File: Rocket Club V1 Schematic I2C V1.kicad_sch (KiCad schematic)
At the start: 8 parts, among them IC1 STM32H573RIT6, J1 USB4135-GF-A_REVA, U1 H3LIS100DLTR, U2 LSM6DSOTR, U3 MAX-M8W-0, U4 MT25TL01GBBB8ESF-0AAT, U5 STLINK-V3MODS

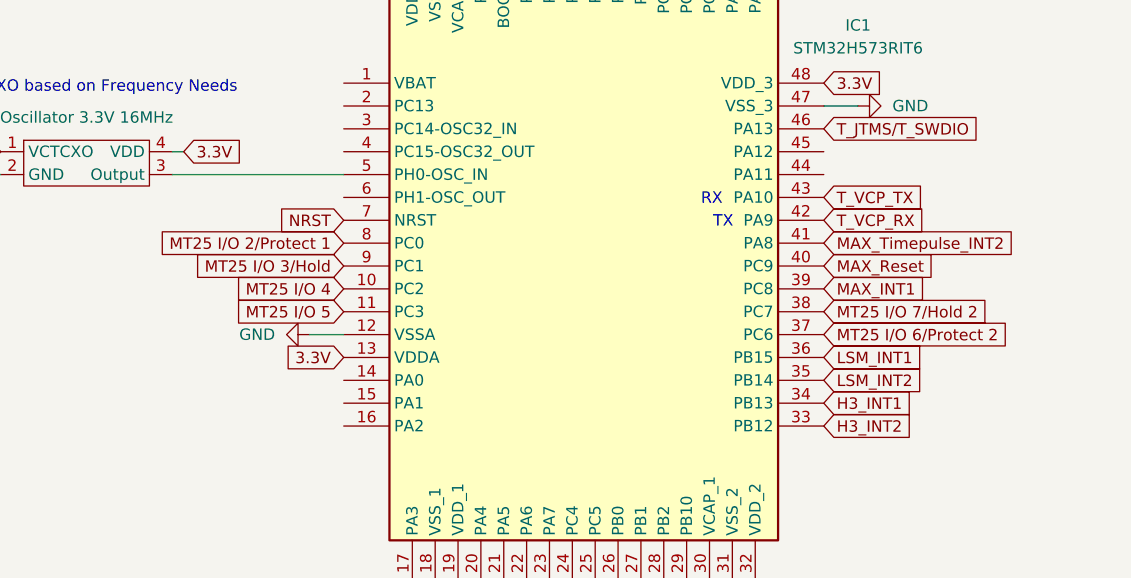
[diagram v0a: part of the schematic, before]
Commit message: Made Sure all labels have an in and an out
Should be labeled to my best extent
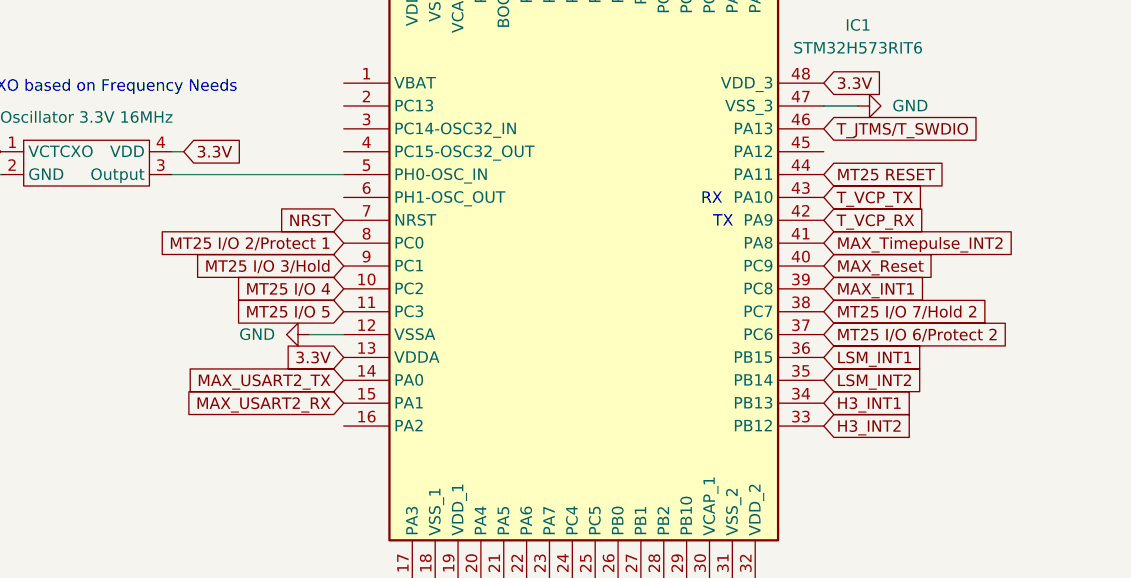
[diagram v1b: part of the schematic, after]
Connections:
- net MAX_USART2_RX: now also IC1.15 (PA1)
- net MAX_USART2_TX: now also IC1.14 (PA0)
- net MT25 RESET: now also IC1.44 (PA11)
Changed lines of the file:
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@@
+		)
+	)
+	(global_label "MAX_USART2_TX"
+		(shape input)
+		(at 250.19 190.5 180)
+		(fields_autoplaced yes)
+		(effects
+			(font
+				(size 1.27 1.27)
+			)
+			(justify right)
+		)
+		(property "Intersheetrefs" "${INTERSHEET_REFS}"
+			(at 232.2673 190.5 0)
+			(effects
+				(font
+					(size 1.27 1.27)
+				)
+				(justify right)
+				(hide yes)
+			)
 		)
 	)
@@
 		)
 	)
+	(global_label "MAX_USART2_RX"
+		(shape input)
+		(at 250.19 193.04 180)
+		(fields_autoplaced yes)
+		(effects
+			(font
+				(size 1.27 1.27)
+			)
+			(justify right)
+		)
+		(property "Intersheetrefs" "${INTERSHEET_REFS}"
+			(at 231.9649 193.04 0)
+			(effects
+				(font
+					(size 1.27 1.27)
+				)
+				(justify right)
+				(hide yes)
+			)
+		)
+	)
 	(global_label "MT25 I{slash}O 7{slash}Hold 2"
 		(shape input)
@@
 		)
 	)
+	(global_label "MT25 RESET"
+		(shape input)
+		(at 303.53 167.64 0)
+		(fields_autoplaced yes)
+		(effects
+			(font
+				(size 1.27 1.27)
+			)
+			(justify left)
+		)
+		(property "Intersheetrefs" "${INTERSHEET_REFS}"
+			(at 318.0659 167.64 0)
+			(effects
+				(font
+					(size 1.27 1.27)
+				)
+				(justify left)
+				(hide yes)
+			)
+		)
+	)
 	(global_label "I2C1_SCL"
 		(shape input)
@@
 		)
 		(property "Intersheetrefs" "${INTERSHEET_REFS}"
-			(at 200.9842 97.79 0)
-			(effects
-				(font
+			(at 199.8352 97.79 0)
+			(effects
+				(font
